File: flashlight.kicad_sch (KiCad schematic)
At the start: 25 parts, among them J1 USB_B_Micro, J2 Conn_01x03_Pin, Q1 HSS2333, Q2 HSS2333, SW1 SW_DIP_x01, U1 LP4054HB5F, U2 MT3608

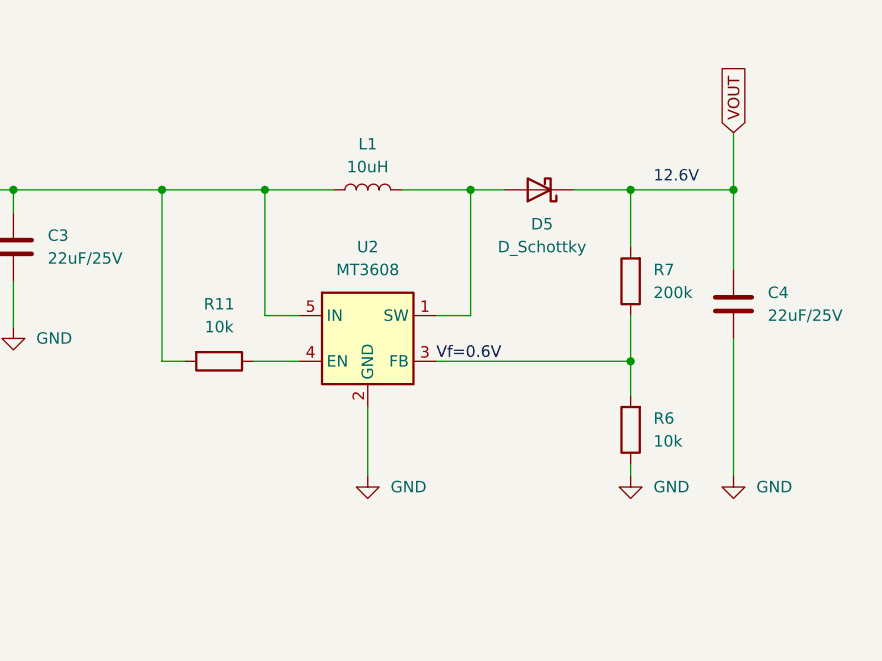
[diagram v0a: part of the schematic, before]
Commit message: tight sot23-6
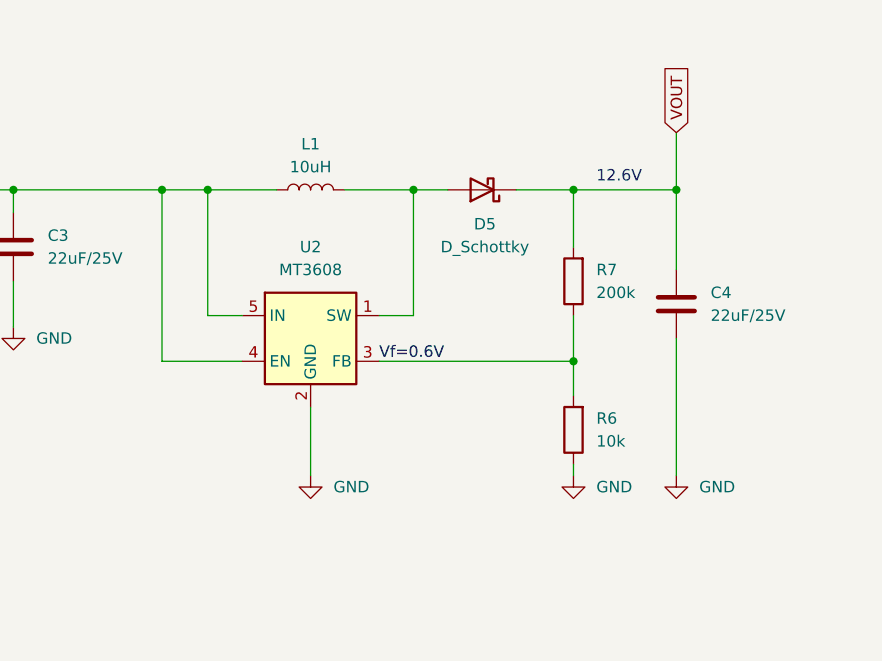
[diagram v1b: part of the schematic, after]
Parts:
- removed R11: 10k, Resistor_SMD:R_0603_1608Metric, symbol Device:R
- U2: footprint Package_TO_SOT_SMD:SOT-23-6 -> SparkFun-Semiconductor-Standard:SOT23-6-Tight
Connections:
- net at C3.1, L1.1, SW1.2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: now also U2.4 (EN)
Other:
- moved on the sheet: C4, D5, L1, R6, R7, U2
